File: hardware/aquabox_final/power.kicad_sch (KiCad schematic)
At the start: 13 parts, among them J1 Entrada de 12V, J2 AC 220V, U1 HLK-10M05

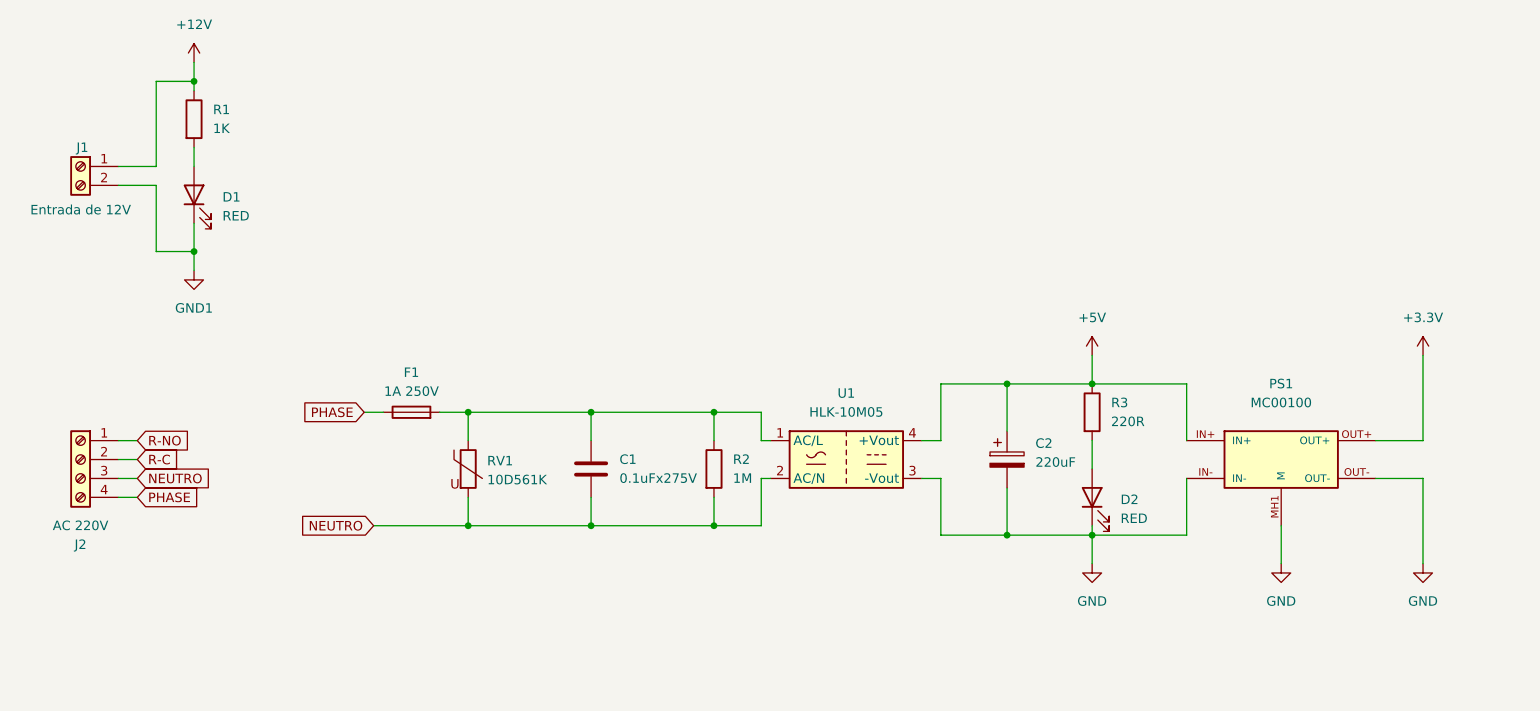
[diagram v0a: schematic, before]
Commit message: Atualização
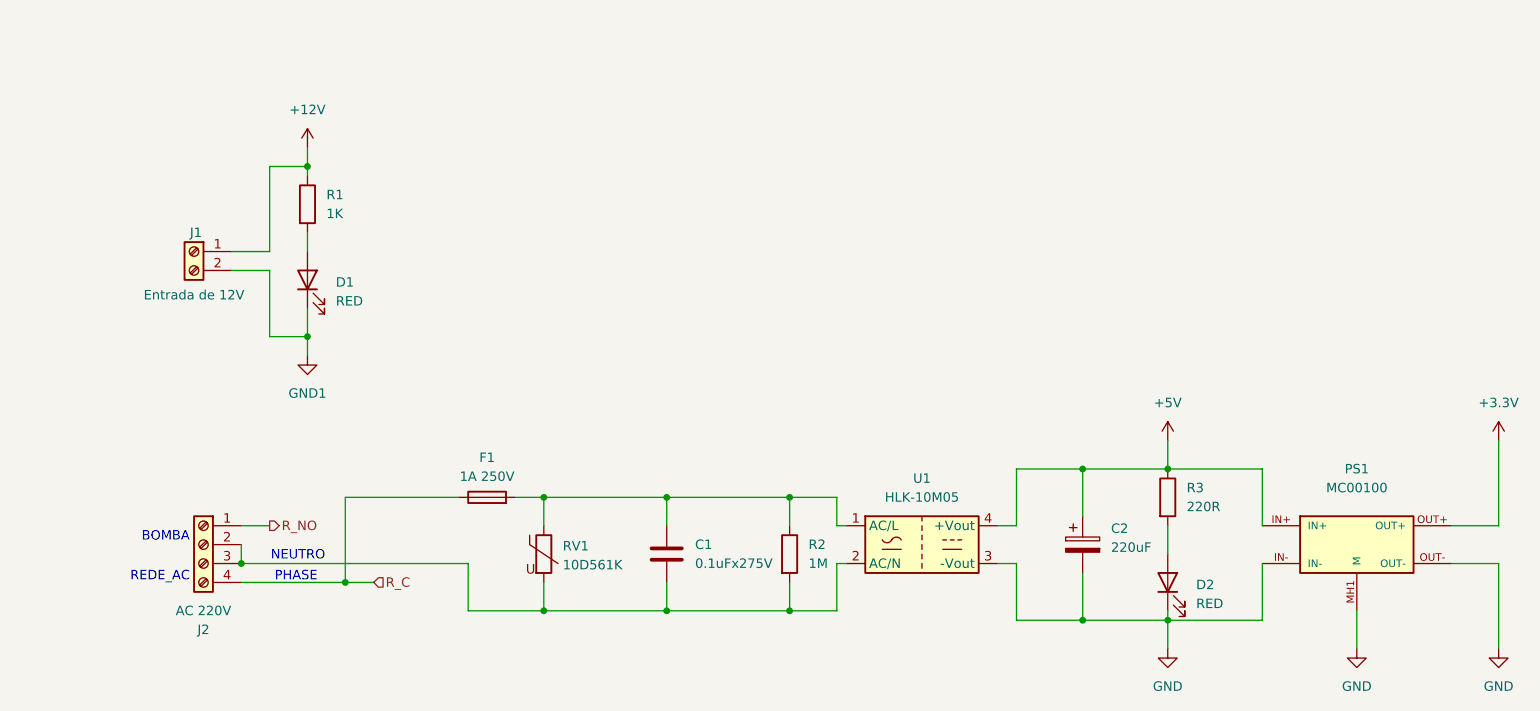
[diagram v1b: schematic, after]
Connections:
- net R-C is gone; now on an unnamed net: J2.2 (Pin_2)
- net NEUTRO: no longer names the net of C1.2, J2.3 (Pin_3), R2.2, RV1.2, U1.2 (AC/N)
- net PHASE renamed R_C
- net R-NO renamed R_NO
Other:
- note added: "BOMBA"
- note added: "NEUTRO"
- note added: "PHASE"
- note added: "REDE_AC"
- moved on the sheet: C1, C2, D1, D2, F1, J1, J2, PS1, R1, R2, R3, RV1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
